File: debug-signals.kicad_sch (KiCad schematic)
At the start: 77 parts

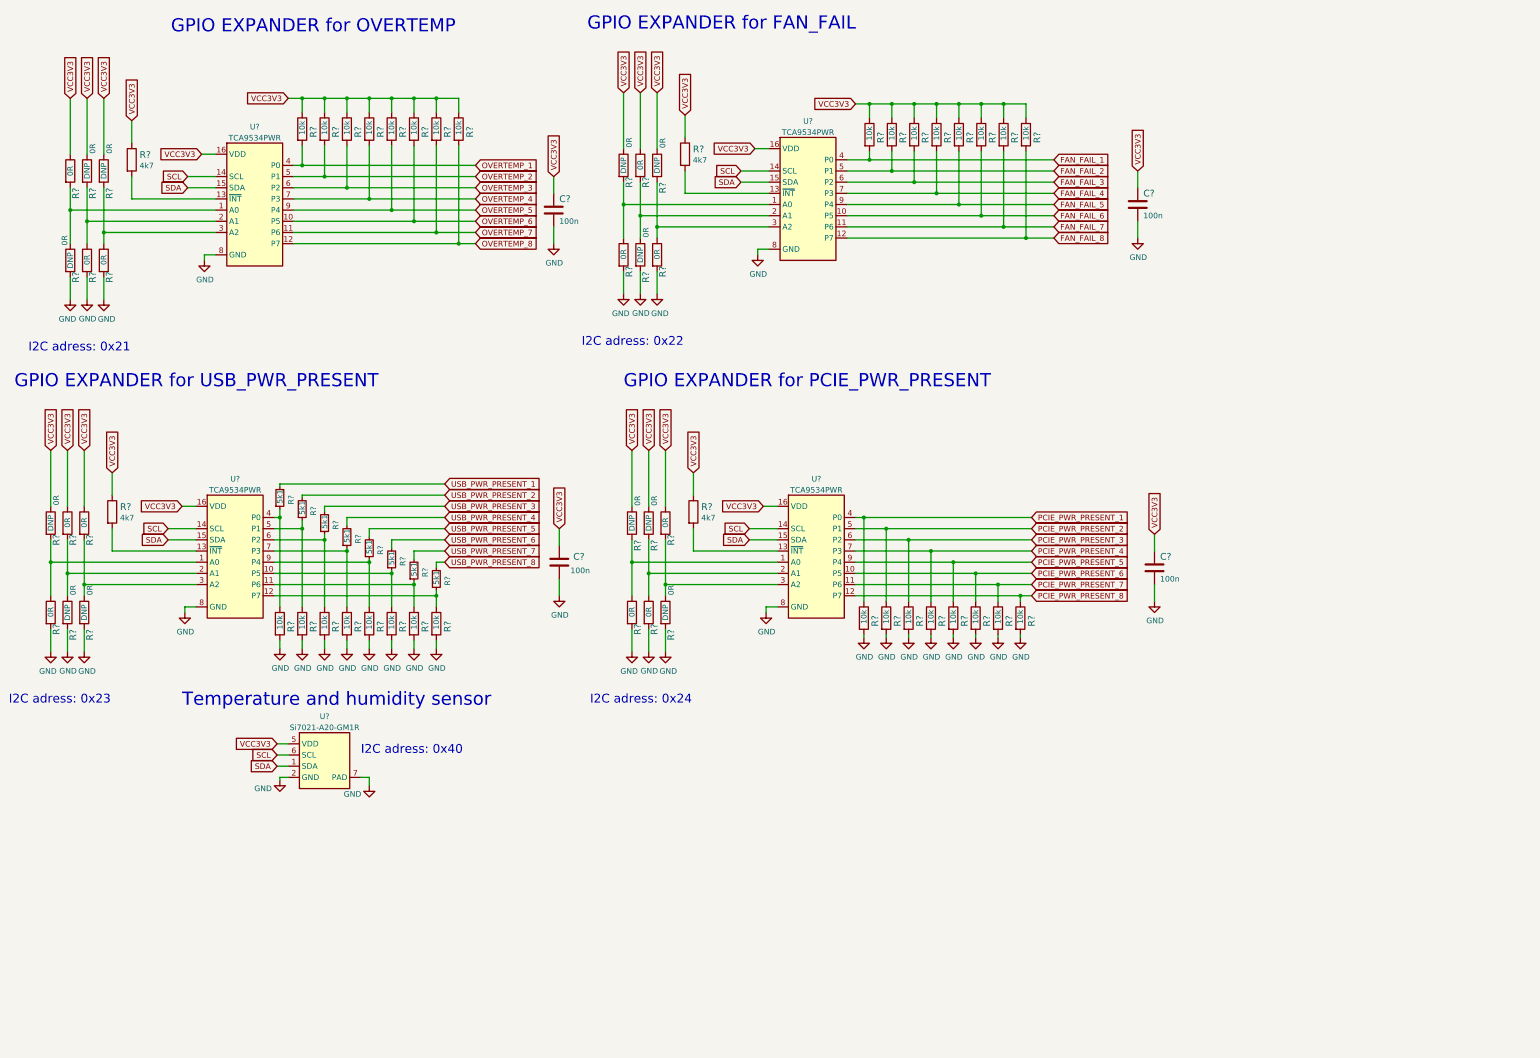
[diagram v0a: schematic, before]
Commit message: Cosmetic changes
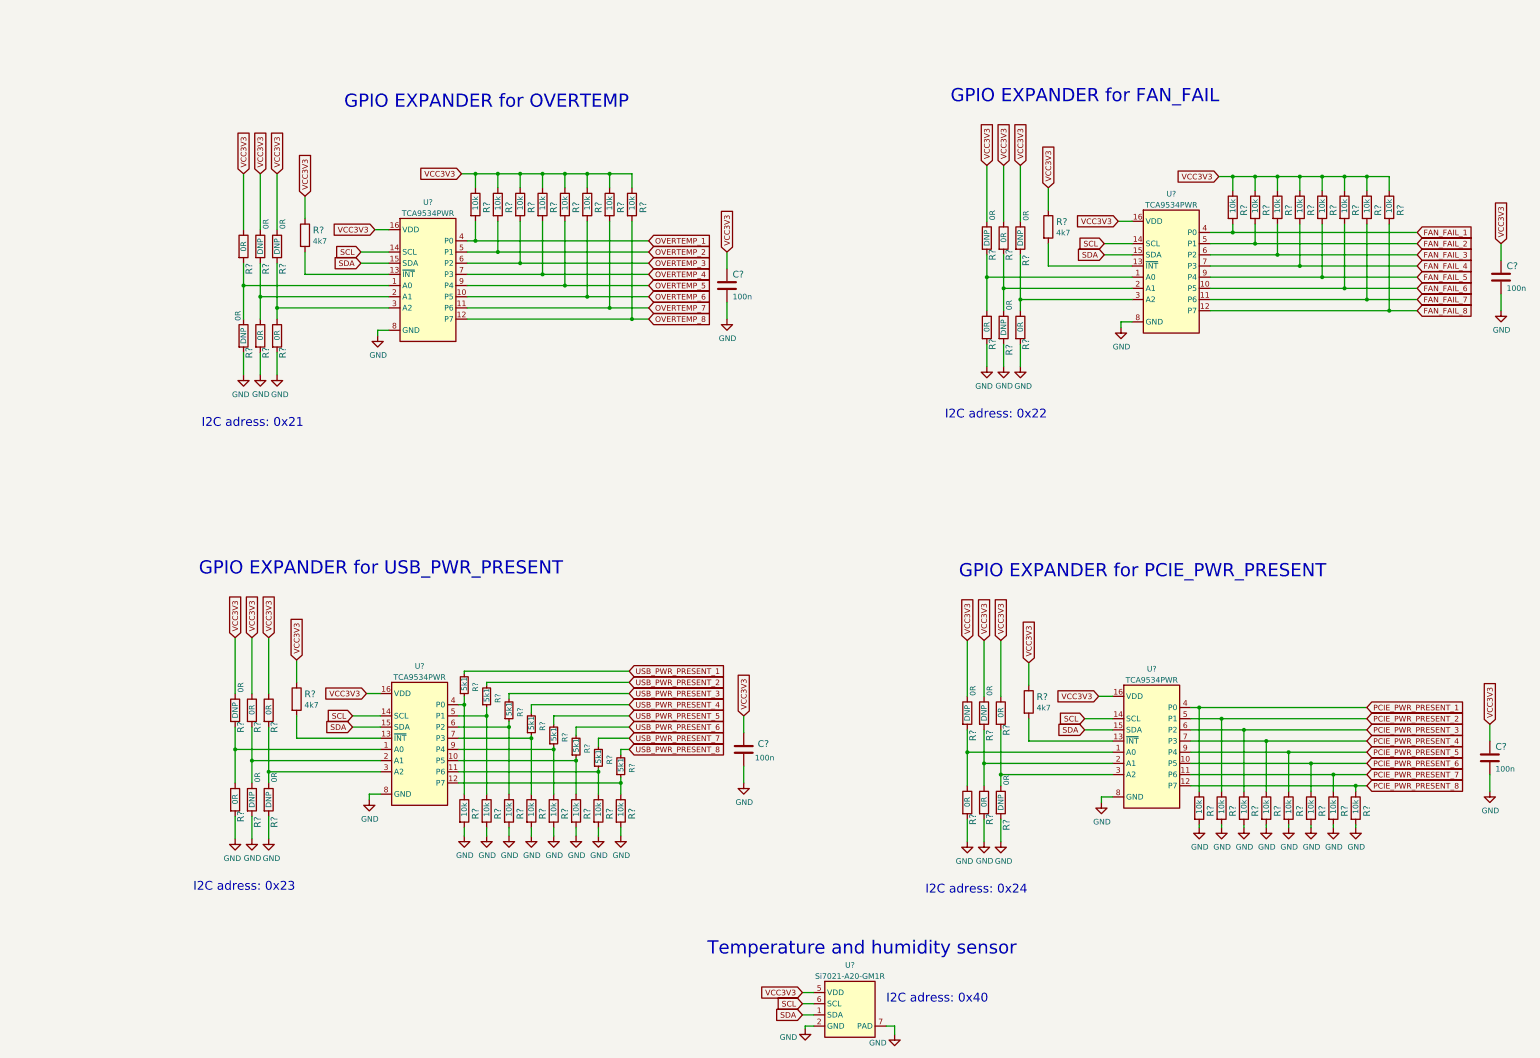
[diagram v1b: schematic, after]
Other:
- moved on the sheet: C?, R?, U?
